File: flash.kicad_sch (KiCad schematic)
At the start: 2 parts, among them U2 W25Q128JVSIQ

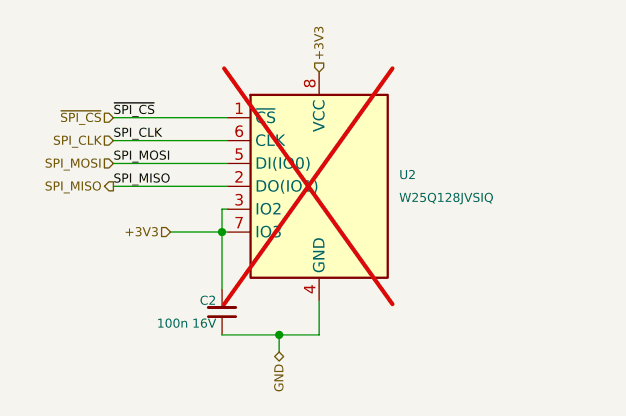
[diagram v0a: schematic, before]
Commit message: WIP
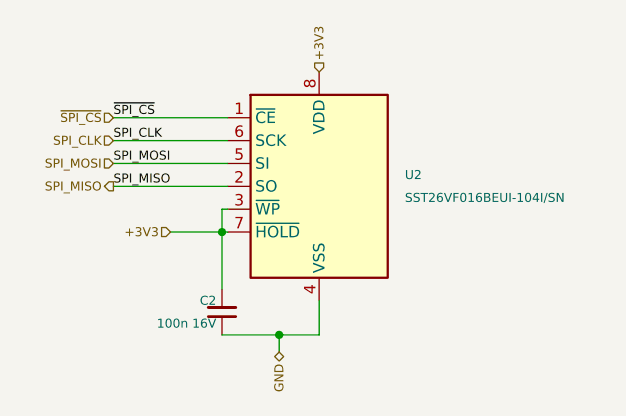
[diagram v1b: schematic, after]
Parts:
- U2: value W25Q128JVSIQ -> SST26VF016BEUI-104I/SN; footprint Package_SO:SOIC-8_5.23x5.23mm_P1.27mm -> Package_SO:SOIC-8_3.9x4.9mm_P1.27mm; symbol Memory_Flash:W25Q32JVSS -> Project_Library:Microchip Technology SST26VF016BEUI-104I/SN; JLCPCB Part # (none) -> C631791; Manufacturer (none) -> Microchip Tech; Partnumber (none) -> SST26VF016BEUI-104I/SN; isBasicPart (none) -> NO; now fitted; now in the parts list
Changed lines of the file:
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@@
     (effects (font (size 1 1)) (justify right))
   )
-  (symbol (lib_id "Memory_Flash:W25Q32JVSS") (at 71.755 34.925 0) (unit 1)
-    (in_bom no) (on_board yes) (dnp yes) (fields_autoplaced)
-    (property "Reference" "U2" (at 80.645 33.655 0)
+  (symbol (lib_id "Project_Library:Microchip Technology SST26VF016BEUI-104I/SN") (at 71.755 34.925 0) (unit 1)
+    (in_bom yes) (on_board yes) (dnp no) (fields_autoplaced)
+    (property "Reference" "U2" (at 81.28 33.6549 0)
       (effects (font (size 1 1)) (justify left))
     )
-    (property "Value" "W25Q128JVSIQ" (at 80.645 36.195 0)
+    (property "Value" "SST26VF016BEUI-104I/SN" (at 81.28 36.1949 0)
       (effects (font (size 1 1)) (justify left))
     )
-    (property "Footprint" "Package_SO:SOIC-8_5.23x5.23mm_P1.27mm" (at 71.755 34.925 0)
-      (effects (font (size 1 1)) hide)
+    (property "Footprint" "Package_SO:SOIC-8_3.9x4.9mm_P1.27mm" (at 71.755 52.705 0)
+      (effects (font (size 1.27 1.27)) hide)
     )
-    (property "Datasheet" "http://www.winbond.com/resource-files/w25q32jv%20revg%2003272018%20plus.pdf" (at 71.755 34.925 0)
-      (effects (font (size 1 1)) hide)
+    (property "Datasheet" "http://ww1.microchip.com/downloads/en/DeviceDoc/20005045C.pdf" (at 71.755 57.785 0)
+      (effects (font (size 1.27 1.27)) hide)
     )
-    (property "Description" "SOP-8-208mil NOR FLASH ROHS" (at 71.755 34.925 0)
-      (effects (font (size 1 1)) hide)
+    (property "Description" "NOR-Flash 16Mbit SPI/SQI Flash w/EUI, 85C, 2.3V-3.6V" (at 71.755 62.865 0)
+      (effects (font (size 1.27 1.27)) hide)
     )
-    (property "Manufacturer" "Winbond Elec" (at 71.755 34.925 0)
-      (effects (font (size 1 1)) hide)
+    (property "Manufacturer" "Microchip Tech" (at 71.755 65.405 0)
+      (effects (font (size 1.27 1.27)) hide)
     )
-    (property "Partnumber" "W25Q128JVSIQ" (at 71.755 34.925 0)
-      (effects (font (size 1 1)) hide)
+    (property "Partnumber" "SST26VF016BEUI-104I/SN" (at 71.755 60.325 0)
+      (effects (font (size 1.27 1.27)) hide)
     )
-    (property "JLCPCB Part #" "C97521" (at 71.755 34.925 0)
-      (effects (font (size 1 1)) hide)
+    (property "JLCPCB Part #" "C631791" (at 71.755 55.245 0) (show_name)
+      (effects (font (size 1.27 1.27)) hide)
     )
-    (property "isBasicPart" "YES" (at 71.755 34.925 0)
-      (effects (font (size 1 1)) hide)
+    (property "isBasicPart" "NO" (at 71.755 67.945 0) (show_name)
+      (effects (font (size 1.27 1.27)) hide)
     )
-    (property "Description" "" (at 71.755 34.925 0)
-      (effects (font (size 1 1)) hide)
+    (property "Description" "NOR-Flash 16Mbit SPI/SQI Flash w/EUI, 85C, 2.3V-3.6V" (at 71.755 62.865 0)
+      (effects (font (size 1.27 1.27)) hide)
     )
-    (property "Manufacturer" "" (at 71.755 34.925 0)
-      (effects (font (size 1 1)) hide)
+    (property "Manufacturer" "Microchip Tech" (at 71.755 65.405 0)
+      (effects (font (size 1.27 1.27)) hide)
     )
-    (property "Partnumber" "" (at 71.755 34.925 0)
-      (effects (font (size 1 1)) hide)
+    (property "Partnumber" "SST26VF016BEUI-104I/SN" (at 71.755 60.325 0)
+      (effects (font (size 1.27 1.27)) hide)
     )
-    (property "JLCPCB Part #" "" (at 71.755 34.925 0)
-      (effects (font (size 1 1)) hide)
+    (property "JLCPCB Part #" "C631791" (at 71.755 55.245 0) (show_name)
+      (effects (font (size 1.27 1.27)) hide)
     )
-    (property "isBasicPart" "" (at 71.755 34.925 0)
-      (effects (font (size 1 1)) hide)
+    (property "isBasicPart" "NO" (at 71.755 67.945 0) (show_name)
+      (effects (font (size 1.27 1.27)) hide)
     )
     (pin "1")
